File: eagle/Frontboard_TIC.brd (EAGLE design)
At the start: 69.8 x 69.8 mm, 21 parts, among them Y1 ABS07-32.768KHZ-7-T, Y2 ABM3B-8.000MHZ-B2-T

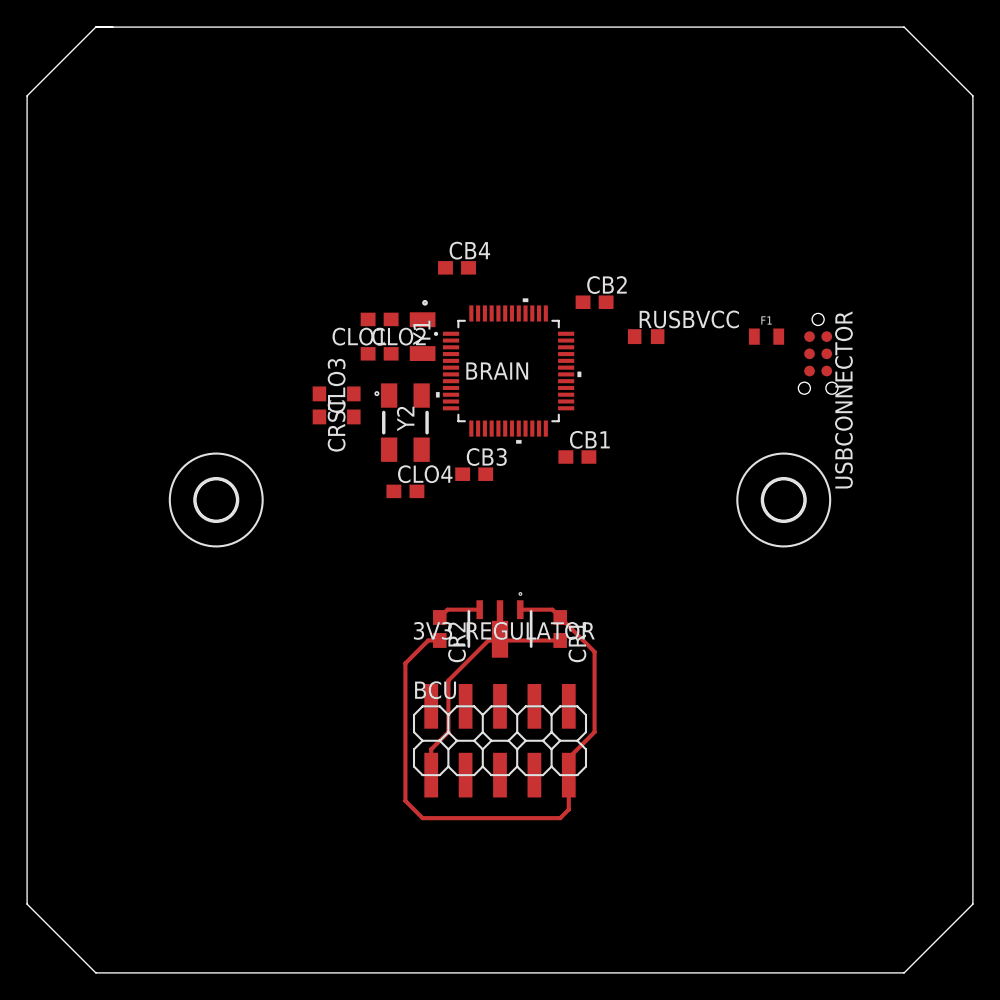
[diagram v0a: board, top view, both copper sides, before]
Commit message: updates
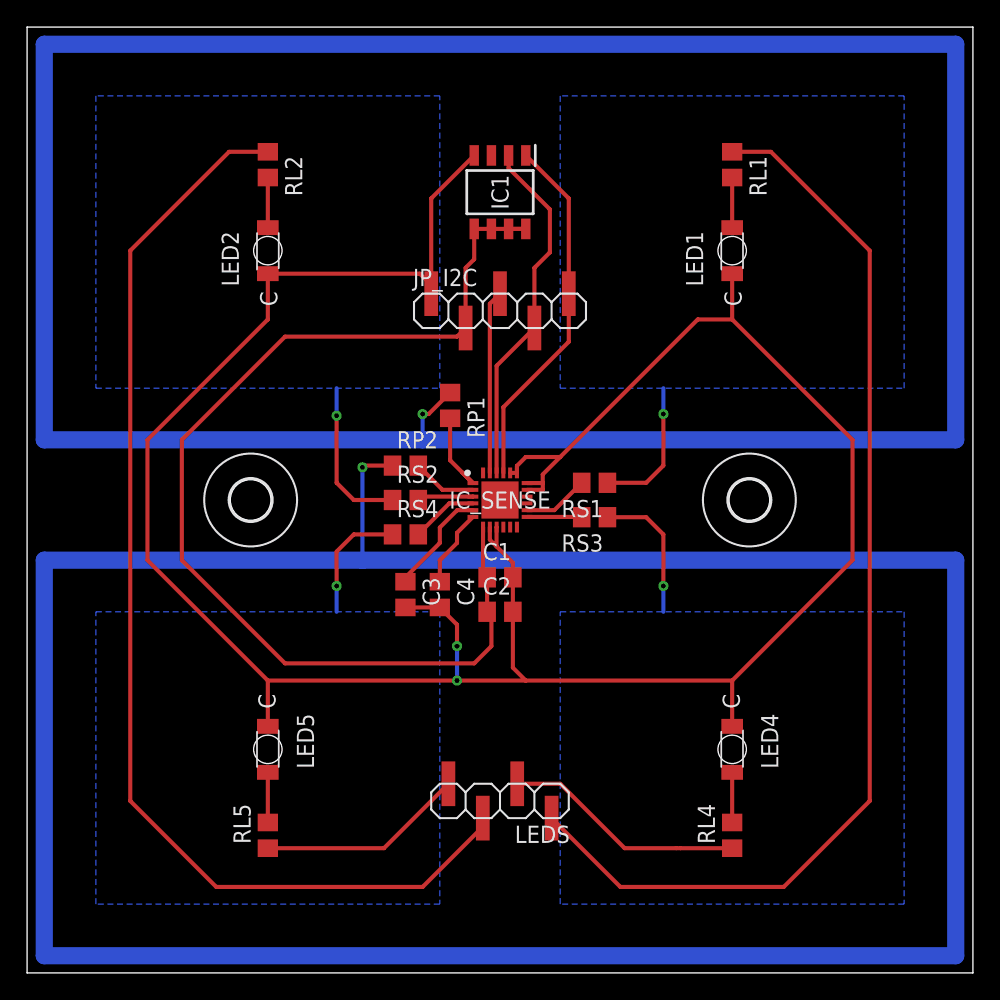
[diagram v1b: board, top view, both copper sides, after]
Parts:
- removed 3V3_REGULATOR: MCP1703T-3302E_MB, MCP1703T-3302E_MB:SOT-89(MB)
- removed BCU: BCU, pinhead:2X05SMD
- removed BRAIN: STM32L072CBT, STM32L072CBT:LQFP48-7X7MM
- removed CB1, CB2, CB3, CB4: 100nf, rcl:C0603
- removed CLO1: 7pF, rcl:C0603
- removed CLO2: 7pf, rcl:C0603
- removed CLO3, CLO4: 18pf, rcl:C0603
- removed CR1, CR2: 1uF, rcl:C0603
- removed CRST: 0.1uF, rcl:C0603
- removed F1: PPTC_6V500MA, SparkFun-Fuses:0805
- removed RUSBVCC: 220, resistor:R0603
- removed USBCONNECTOR: (no value), tag-connect:TC2030-MCP-NL
- removed Y1: ABS07-32.768KHZ-7-T, ABS07-32.768KHZ-7-T:ABS-07
- removed Y2: ABM3B-8.000MHZ-B2-T, ABM3B-8.000MHZ-B2-T:ABM3B
- added C1, C4: 0.1uf, rcl:C0805
- added C2: 1uf, rcl:C0805
- added C3: 2.2nf, rcl:C0805
- added IC1: NCT75DR2G, NCT75DR2G:SOIC127P600X175-8N
- added IC_SENSE: CY8CMBR3116-LQXIT, CY8CMBR3116-LQXIT:QFN50P400X400X60-25N
- added JP_I2C: I2C, pinhead:1X05SMD
- added LED1, LED2, LED4, LED5: WL-SMRW156120BS75300-B_RVS-MOUNT, Wurth_Elektronik_Optoelectronics_rev15b (1):WL-SMRW-1206-CYLDR-REVERSE-MOUNT
- added LEDS: LEDS, pinhead:1X04SMD
- added RL1, RL2, RL4, RL5: 330E, resistor:R0805
- added RP1, RP2, RS1, RS2, RS3, RS4: 560E, resistor:R0805
- moved U$1 2.54 mm to (16.5, 34.9)
- moved U$2 2.54 mm to (53.3, 34.9)
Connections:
- removed net +3V3: 3V3_REGULATOR.3, BRAIN.1, BRAIN.24, BRAIN.48, BRAIN.9, CB1.1, CB2.1, CB3.1, CB4.1, CR2.1
- removed net +5V: 3V3_REGULATOR.2, 3V3_REGULATOR.4, BCU.1, CR1.2
- removed net OSC32_IN: BRAIN.3, CLO1.2, Y1.1
- removed net OSC32_OUT: BRAIN.4, CLO2.2, Y1.2
- removed net OSC_IN: BRAIN.5, CLO3.2, Y2.1
- removed net OSC_OUT: BRAIN.6, CLO4.2, Y2.3
- removed net PA10: BRAIN.31
- removed net PB3: BRAIN.39
- removed net PB4: BRAIN.40
- removed net RXD: BCU.7
- removed net TXD: BCU.3
- removed net USB_DM: BRAIN.32, USBCONNECTOR.5
- removed net USB_DP: BRAIN.33, USBCONNECTOR.4
- removed net USB_VCC: BRAIN.36, RUSBVCC.1
- new net HOST_INT: IC_SENSE.23, JP_I2C.3
- new net I2C_SCL: IC1.2, IC_SENSE.22, JP_I2C.4
- new net I2C_SDA: IC1.1, IC_SENSE.21, JP_I2C.5
- new net LED1: LEDS.1, RL1.1
- new net LED2: LEDS.3, RL2.1
- new net LED4: LEDS.2, RL4.1
- new net LED5: LEDS.4, RL5.1
- new net N$10: LED5.2, RL5.2
- new net N$19: C4.1, IC_SENSE.6
- new net N$20: C3.1, IC_SENSE.5
- new net N$4: IC_SENSE.13, RS3.2
- new net N$5: IC_SENSE.1, RP1.2
- new net N$6: IC_SENSE.2, RP2.2
- new net N$7: IC_SENSE.4, RS4.2
- new net N$8: IC_SENSE.3, RS2.2
- new net N$9: LED4.2, RL4.2
- new net SENS_1: RS1.1
- new net SENS_2: RS2.1
- new net SENS_3: RS3.1
- new net SENS_4: RS4.1
- new net SENS_PROX_1: RP1.1
- new net SENS_PROX_2: RP2.1
- new net VCC: C1.1, C2.1, IC1.5, IC1.6, IC1.7, IC1.8, IC_SENSE.7, JP_I2C.2
- net GND: now also C1.2, C2.2, C3.2, C4.2, IC1.4, IC_SENSE.17, IC_SENSE.18, IC_SENSE.19, IC_SENSE.20, IC_SENSE.8, IC_SENSE.9, JP_I2C.1, LED1.1, LED2.1, LED4.1, LED5.1; no longer 3V3_REGULATOR.1, BCU.9, BRAIN.23, BRAIN.35, BRAIN.44, BRAIN.47, BRAIN.8, CB1.2, CB2.2, CB3.2, CB4.2, CLO1.1, CLO2.1, CLO3.1, CLO4.1, CR1.1, CR2.2, CRST.2, USBCONNECTOR.3, Y2.2, Y2.4
- net N$1: now also LED1.2, RL1.2; no longer BRAIN.7, CRST.1
- net N$2: now also LED2.2, RL2.2; no longer F1.2, USBCONNECTOR.2
- net N$3: now also IC_SENSE.14, RS1.2; no longer F1.1, RUSBVCC.2
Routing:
- net SENS_PROX_2: track 0.00 -> 202.3 mm, vias 0 -> 1
- net SENS_PROX_1: track 0.00 -> 197.6 mm, vias 0 -> 1
- net GND: track 45.5 -> 188.9 mm, vias 0 -> 2
- net LED2: track 0.00 -> 85.0 mm
- net VCC: track 0.00 -> 82.4 mm
- net LED1: track 0.00 -> 82.1 mm
- net I2C_SCL: track 0.00 -> 27.0 mm
- net I2C_SDA: track 0.00 -> 26.8 mm
- net +5V: track 19.2 -> 0.00 mm
- net LED4: track 0.00 -> 17.8 mm
- net LED5: track 0.00 -> 15.3 mm
- net HOST_INT: track 0.00 -> 13.6 mm
- net SENS_2: track 0.00 -> 11.6 mm, vias 0 -> 1
- net SENS_3: track 0.00 -> 10.4 mm, vias 0 -> 1
- net SENS_1: track 0.00 -> 10.4 mm, vias 0 -> 1
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- added copper zone on layer 16, net SENS_1
- added copper zone on layer 16, net SENS_2
- added copper zone on layer 16, net SENS_3
- added copper zone on layer 16, net SENS_4
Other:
- outline, holes or cut-outs redrawn
